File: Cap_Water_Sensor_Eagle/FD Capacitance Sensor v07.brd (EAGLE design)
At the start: 160 x 100 mm, 17 parts, among them U1 NTS4101PT1, U2 TLC555CD

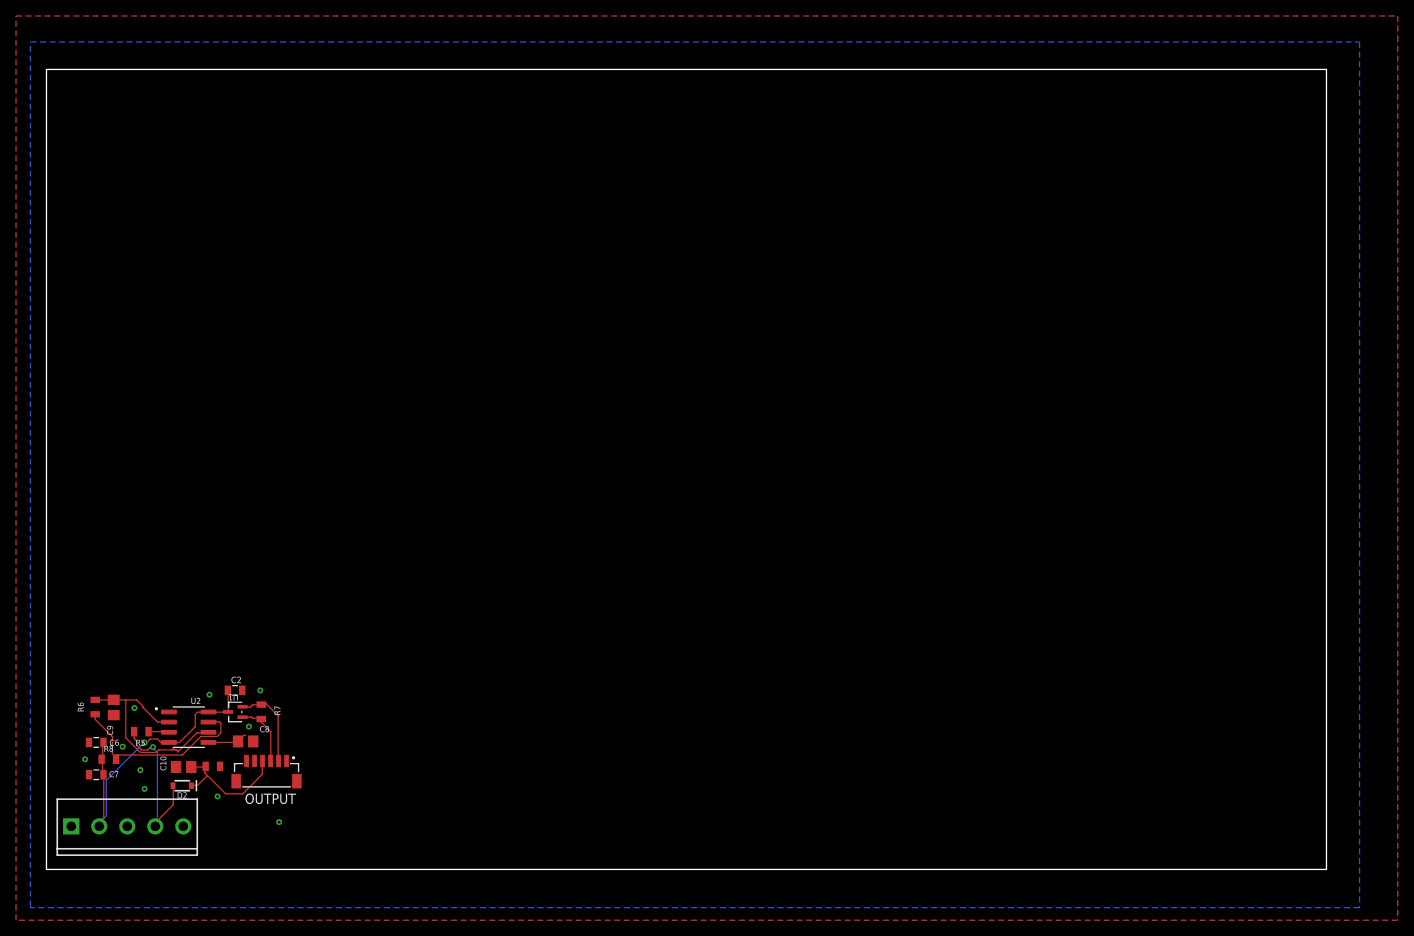
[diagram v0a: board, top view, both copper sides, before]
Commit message: FIGURED OUT STUFF
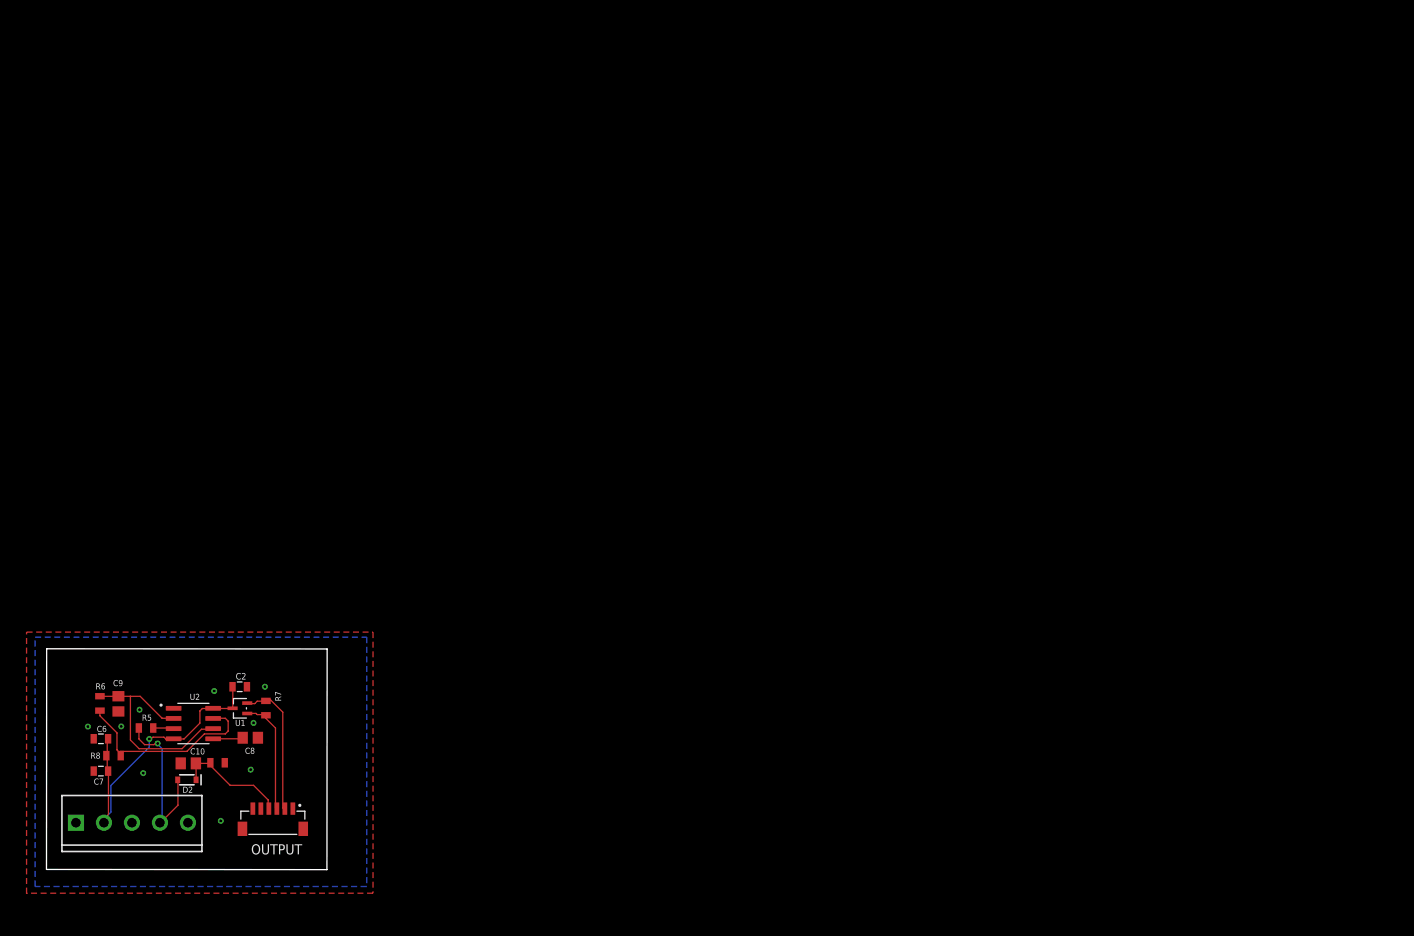
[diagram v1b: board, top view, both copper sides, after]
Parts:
- moved FRAME1 72.0 mm to (-1.55, -6.20)
- moved OUTPUT 6.00 mm to (28.3, 5.08)
- moved D2 0.94 mm to (17.6, 11.2)
- moved U1 0.74 mm to (24.2, 20.1)
- moved C6 0.74 mm to (6.81, 16.3)
- moved C7 0.74 mm to (6.81, 12.3)
- moved R6 0.74 mm to (6.68, 20.8)
- moved R8 0.74 mm to (8.38, 14.2)
- moved C10 0.74 mm to (17.7, 13.3)
- moved C8 0.74 mm to (25.5, 16.5)
- moved C9 0.74 mm to (8.99, 20.7)
- moved R5 0.74 mm to (12.4, 17.7)
- moved R7 0.74 mm to (27.4, 20.2)
- moved R9 0.74 mm to (21.4, 13.3)
- moved U2 0.74 mm to (18.4, 18.2)
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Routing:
- net +3V3: track 11.0 -> 17.6 mm
- net !EN: track 8.26 -> 14.8 mm
- net OUTPUT1: track 17.2 -> 15.3 mm
- net N$1: track 5.04 -> 3.79 mm
- net N$9: track 24.3 -> 25.0 mm
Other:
- board size 160 x 100 mm -> 35.1 x 27.6 mm
